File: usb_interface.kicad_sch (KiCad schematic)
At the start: 55 parts, among them J7 GCT USB4105-GF-A-120, J8 PD_I2C DEBUG, Q1 CSD25480F3, Q2 CSD15380F3, Q3 CSD25480F3, Q4 CSD15380F3, U3 TVS2200DRV, U4 TPD8S300/A, U5 TI TPS25751DREFR, U6 CAT24C256

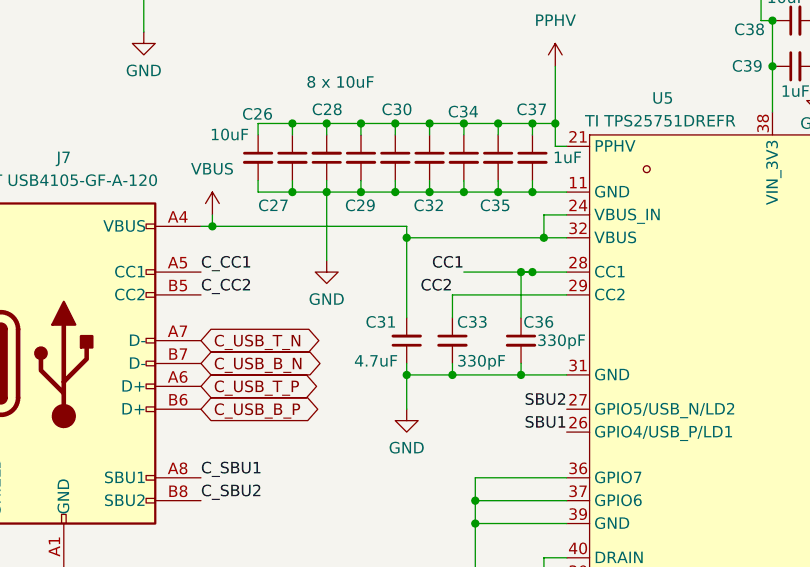
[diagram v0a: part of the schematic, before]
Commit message: done pcb layout
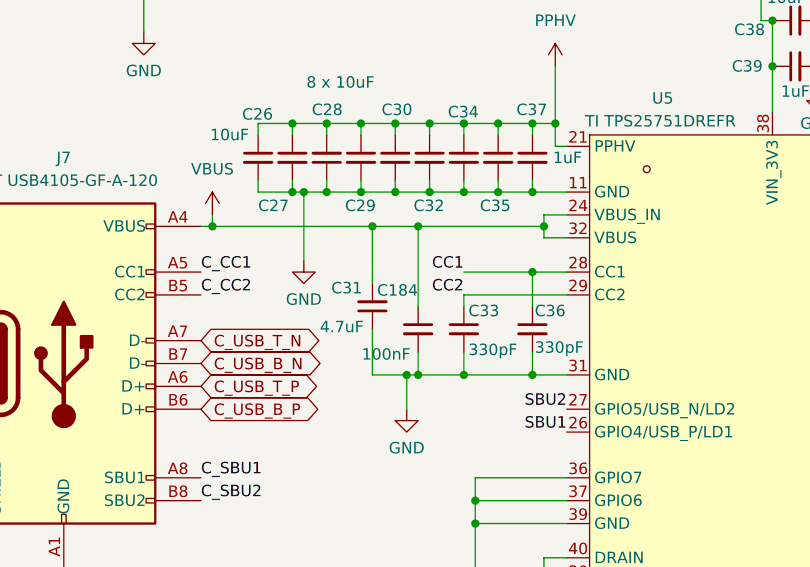
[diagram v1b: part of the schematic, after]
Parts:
- added C184: 100nF, Capacitor_SMD:C_0402_1005Metric, symbol Device:C_Small
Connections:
- net GND: now also C184.2
- net VBUS: now also C184.1
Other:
- company: Ryan Di Lorenzo -> LimesKey
- moved on the sheet: C31, C33, C36

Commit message: add 3d models locally
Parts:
- U6: footprint Package_DFN_QFN:OnSemi_UDFN-8_1.2x1.8mm_P0.4mm -> Package_DFN_QFN:DFN-8-1EP_2x3mm_P0.5mm_EP0.61x2.2mm
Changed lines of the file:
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@@
 			)
 		)
-		(property "Footprint" "Package_DFN_QFN:OnSemi_UDFN-8_1.2x1.8mm_P0.4mm"
+		(property "Footprint" "Package_DFN_QFN:DFN-8-1EP_2x3mm_P0.5mm_EP0.61x2.2mm"
 			(at 243.84 90.17 0)
 			(hide yes)
